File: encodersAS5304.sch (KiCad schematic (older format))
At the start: 5 parts, among them P101 CONN_01X02, P102 CONN_01X02, U101 AS5304

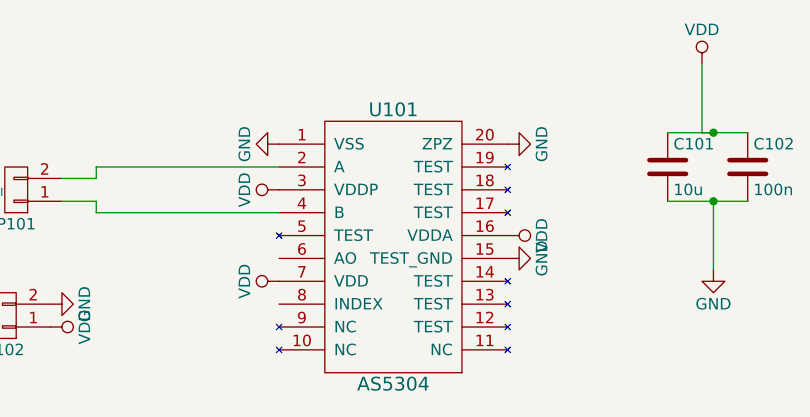
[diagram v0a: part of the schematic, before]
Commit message: pcb
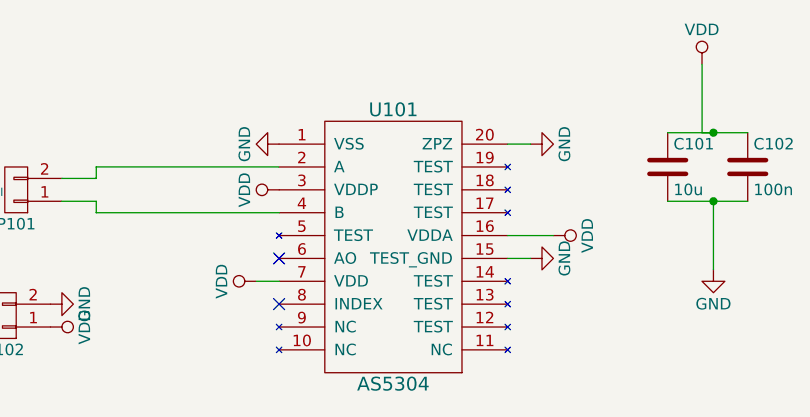
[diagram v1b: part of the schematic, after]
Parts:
- C101, C102: footprint (none) -> Capacitors_SMD:C_1210_HandSoldering
- P101, P102: footprint (none) -> Pin_Headers:Pin_Header_Straight_1x02
- U101: footprint (none) -> Housings_SSOP:SSOP-20_4.4x6.5mm_Pitch0.65mm
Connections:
- no-connect marks 0 -> 2
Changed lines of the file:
@@
 LIBS:valves
 LIBS:as5304
+LIBS:encodersAS5304-cache
 EELAYER 25 0
 EELAYER END
@@
 F 0 "U101" H 5400 3800 60  0000 C CNN
 F 1 "AS5304" H 5400 2600 60  0000 C CNN
-F 2 "" H 5400 3200 60  0000 C CNN
+F 2 "Housings_SSOP:SSOP-20_4.4x6.5mm_Pitch0.65mm" H 5400 3200 60  0001 C CNN
 F 3 "" H 5400 3200 60  0000 C CNN
 	1    5400 3200
@@
 F 0 "P101" H 3750 3100 50  0000 C CNN
 F 1 "CONN_01X02" V 3850 2950 50  0000 C CNN
-F 2 "" H 3750 2950 50  0000 C CNN
+F 2 "Pin_Headers:Pin_Header_Straight_1x02" H 3750 2950 50  0001 C CNN
 F 3 "" H 3750 2950 50  0000 C CNN
 	1    3750 2950
@@
 	4100 3000 3950 3000
 $Comp
-L GND #PWR106
+L GND #PWR01
 U 1 1 5823612A
-P 5900 2750
-F 0 "#PWR106" H 5900 2500 50  0001 C CNN
-F 1 "GND" H 5900 2600 50  0000 C CNN
-F 2 "" H 5900 2750 50  0000 C CNN
-F 3 "" H 5900 2750 50  0000 C CNN
-	1    5900 2750
-	0    -1   -1   0
-$EndComp
-$Comp
-L GND #PWR103
+P 6000 2750
+F 0 "#PWR01" H 6000 2500 50  0001 C CNN
+F 1 "GND" H 6000 2600 50  0000 C CNN
+F 2 "" H 6000 2750 50  0000 C CNN
+F 3 "" H 6000 2750 50  0000 C CNN
+	1    6000 2750
+	0    -1   -1   0
+$EndComp
+$Comp
+L GND #PWR02
 U 1 1 58236142
 P 4900 2750
-F 0 "#PWR103" H 4900 2500 50  0001 C CNN
+F 0 "#PWR02" H 4900 2500 50  0001 C CNN
 F 1 "GND" H 4900 2600 50  0000 C CNN
 F 2 "" H 4900 2750 50  0000 C CNN
@@
 $EndComp
 $Comp
-L GND #PWR108
+L GND #PWR03
 U 1 1 58236169
-P 5900 3250
-F 0 "#PWR108" H 5900 3000 50  0001 C CNN
-F 1 "GND" H 5900 3100 50  0000 C CNN
-F 2 "" H 5900 3250 50  0000 C CNN
-F 3 "" H 5900 3250 50  0000 C CNN
-	1    5900 3250
-	0    -1   -1   0
-$EndComp
-$Comp
-L VDD #PWR107
+P 6000 3250
+F 0 "#PWR03" H 6000 3000 50  0001 C CNN
+F 1 "GND" H 6000 3100 50  0000 C CNN
+F 2 "" H 6000 3250 50  0000 C CNN
+F 3 "" H 6000 3250 50  0000 C CNN
+	1    6000 3250
+	0    -1   -1   0
+$EndComp
+$Comp
+L VDD #PWR04
 U 1 1 58236181
-P 5900 3150
-F 0 "#PWR107" H 5900 3000 50  0001 C CNN
-F 1 "VDD" H 5900 3300 50  0000 C CNN
-F 2 "" H 5900 3150 50  0000 C CNN
-F 3 "" H 5900 3150 50  0000 C CNN
-	1    5900 3150
+P 6100 3150
+F 0 "#PWR04" H 6100 3000 50  0001 C CNN
+F 1 "VDD" H 6100 3300 50  0000 C CNN
+F 2 "" H 6100 3150 50  0000 C CNN
+F 3 "" H 6100 3150 50  0000 C CNN
+	1    6100 3150
 	0    1    1    0
 $EndComp
 $Comp
-L VDD #PWR104
+L VDD #PWR05
 U 1 1 58236199
 P 4900 2950
-F 0 "#PWR104" H 4900 2800 50  0001 C CNN
+F 0 "#PWR05" H 4900 2800 50  0001 C CNN
 F 1 "VDD" H 4900 3100 50  0000 C CNN
 F 2 "" H 4900 2950 50  0000 C CNN
@@
 $EndComp
 $Comp
-L VDD #PWR105
+L VDD #PWR06
 U 1 1 582361B1
-P 4900 3350
-F 0 "#PWR105" H 4900 3200 50  0001 C CNN
-F 1 "VDD" H 4900 3500 50  0000 C CNN
-F 2 "" H 4900 3350 50  0000 C CNN
-F 3 "" H 4900 3350 50  0000 C CNN
-	1    4900 3350
-	0    -1   -1   0
-$EndComp
-$Comp
-L VDD #PWR109
+P 4800 3350
+F 0 "#PWR06" H 4800 3200 50  0001 C CNN
+F 1 "VDD" H 4800 3500 50  0000 C CNN
+F 2 "" H 4800 3350 50  0000 C CNN
+F 3 "" H 4800 3350 50  0000 C CNN
+	1    4800 3350
+	0    -1   -1   0
+$EndComp
+$Comp
+L VDD #PWR07
 U 1 1 582361C9
 P 6750 2400
-F 0 "#PWR109" H 6750 2250 50  0001 C CNN
+F 0 "#PWR07" H 6750 2250 50  0001 C CNN
 F 1 "VDD" H 6750 2550 50  0000 C CNN
 F 2 "" H 6750 2400 50  0000 C CNN
@@
 $EndComp
 $Comp
-L GND #PWR110
+L GND #PWR08
 U 1 1 582361E1
 P 6800 3300
-F 0 "#PWR110" H 6800 3050 50  0001 C CNN
+F 0 "#PWR08" H 6800 3050 50  0001 C CNN
 F 1 "GND" H 6800 3150 50  0000 C CNN
 F 2 "" H 6800 3300 50  0000 C CNN
@@
 F 0 "C101" H 6625 2950 50  0000 L CNN
 F 1 "10u" H 6625 2750 50  0000 L CNN
-F 2 "" H 6638 2700 50  0000 C CNN
+F 2 "Capacitors_SMD:C_1210_HandSoldering" H 6638 2700 50  0001 C CNN
 F 3 "" H 6600 2850 50  0000 C CNN
 	1    6600 2850
@@
 F 0 "C102" H 6975 2950 50  0000 L CNN
 F 1 "100n" H 6975 2750 50  0000 L CNN
-F 2 "" H 6988 2700 50  0000 C CNN
+F 2 "Capacitors_SMD:C_1210_HandSoldering" H 6988 2700 50  0001 C CNN
 F 3 "" H 6950 2850 50  0000 C CNN
 	1    6950 2850
@@
 F 0 "P102" H 3700 3650 50  0000 C CNN
 F 1 "CONN_01X02" V 3800 3500 50  0000 C CNN
-F 2 "" H 3700 3500 50  0000 C CNN
+F 2 "Pin_Headers:Pin_Header_Straight_1x02" H 3700 3500 50  0001 C CNN
 F 3 "" H 3700 3500 50  0000 C CNN
 	1    3700 3500
@@
 $EndComp
 $Comp
-L GND #PWR101
+L GND #PWR09
 U 1 1 58236307
 P 3900 3450
-F 0 "#PWR101" H 3900 3200 50  0001 C CNN
+F 0 "#PWR09" H 3900 3200 50  0001 C CNN
 F 1 "GND" H 3900 3300 50  0000 C CNN
 F 2 "" H 3900 3450 50  0000 C CNN
@@
 $EndComp
 $Comp
-L VDD #PWR102
+L VDD #PWR010
 U 1 1 58236325
 P 3900 3550
-F 0 "#PWR102" H 3900 3400 50  0001 C CNN
+F 0 "#PWR010" H 3900 3400 50  0001 C CNN
 F 1 "VDD" H 3900 3700 50  0000 C CNN
 F 2 "" H 3900 3550 50  0000 C CNN
@@
 	0    1    1    0
 $EndComp
+NoConn ~ 4900 3250
+NoConn ~ 4900 3450
+Wire Wire Line
+	6000 2750 5900 2750
+Wire Wire Line
+	6100 3150 5900 3150
+Wire Wire Line
+	6000 3250 5900 3250
+Wire Wire Line
+	4900 3350 4800 3350
 $EndSCHEMATC

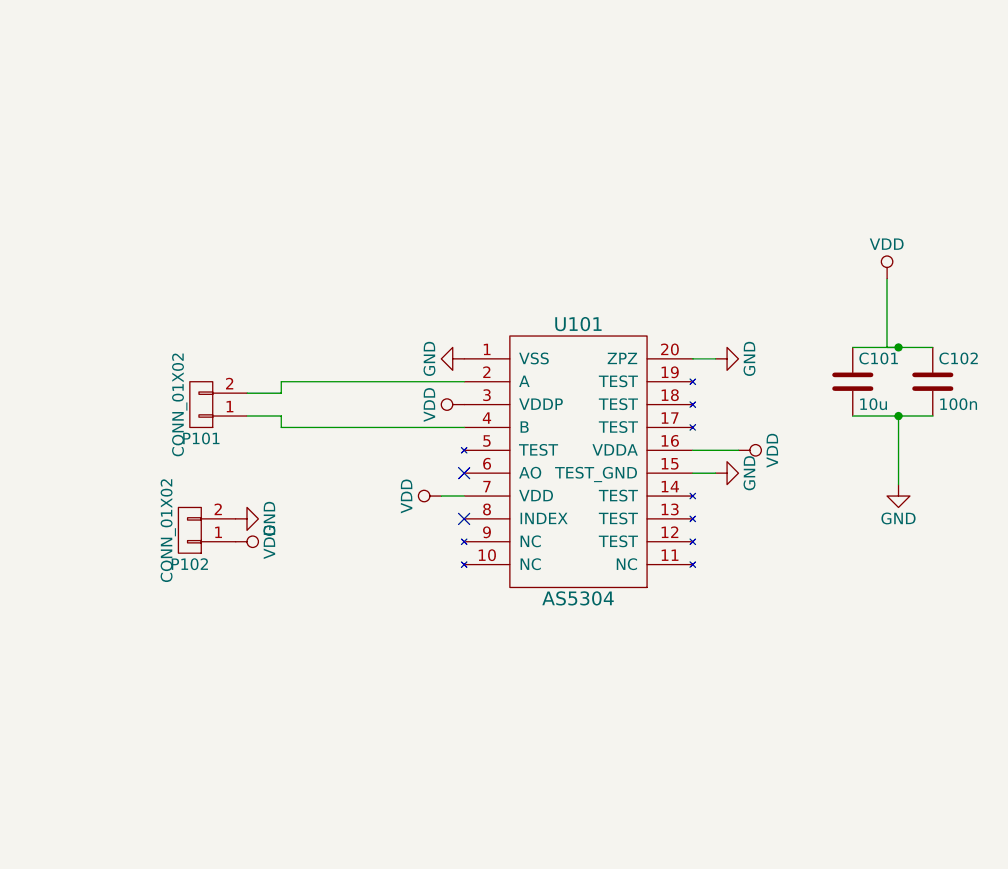
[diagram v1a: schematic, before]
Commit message: placa con forma apropiada y dimensiones exactas. Falta enrutado
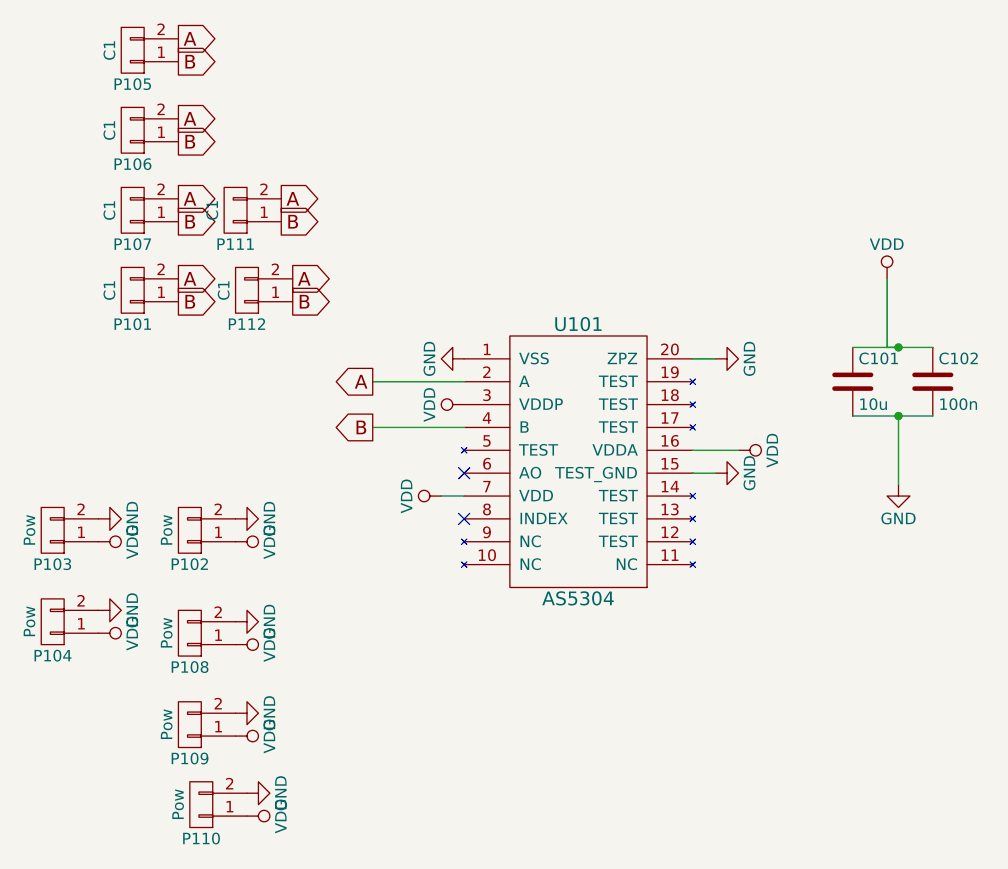
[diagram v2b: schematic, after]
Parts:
- added P103, P104, P108, P109, P110: Pow, Pin_Headers:Pin_Header_Straight_1x02, symbol CONN_01X02
- added P105, P106, P107, P111, P112: C1, Pin_Headers:Pin_Header_Straight_1x02, symbol CONN_01X02
- P101: value CONN_01X02 -> C1
- P102: value CONN_01X02 -> Pow
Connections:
- net GND: now also P103.2 (P2), P104.2 (P2), P108.2 (P2), P109.2 (P2), P110.2 (P2)
- net VDD: now also P103.1 (P1), P104.1 (P1), P108.1 (P1), P109.1 (P1), P110.1 (P1)
- net A: now reaches P101.2 (P2), U101.2 (A)
- net A: now also P105.2 (P2), P106.2 (P2), P107.2 (P2), P111.2 (P2), P112.2 (P2)
- net B: now reaches P101.1 (P1), U101.4 (B)
- net B: now also P105.1 (P1), P106.1 (P1), P107.1 (P1), P111.1 (P1), P112.1 (P1)
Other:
- moved on the sheet: P101
